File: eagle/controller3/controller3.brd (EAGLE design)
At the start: 68.6 x 63.5 mm, 55 parts, among them J4 USB-MICROB, Q3 MOSFET-NCHANNELFQP30N06L

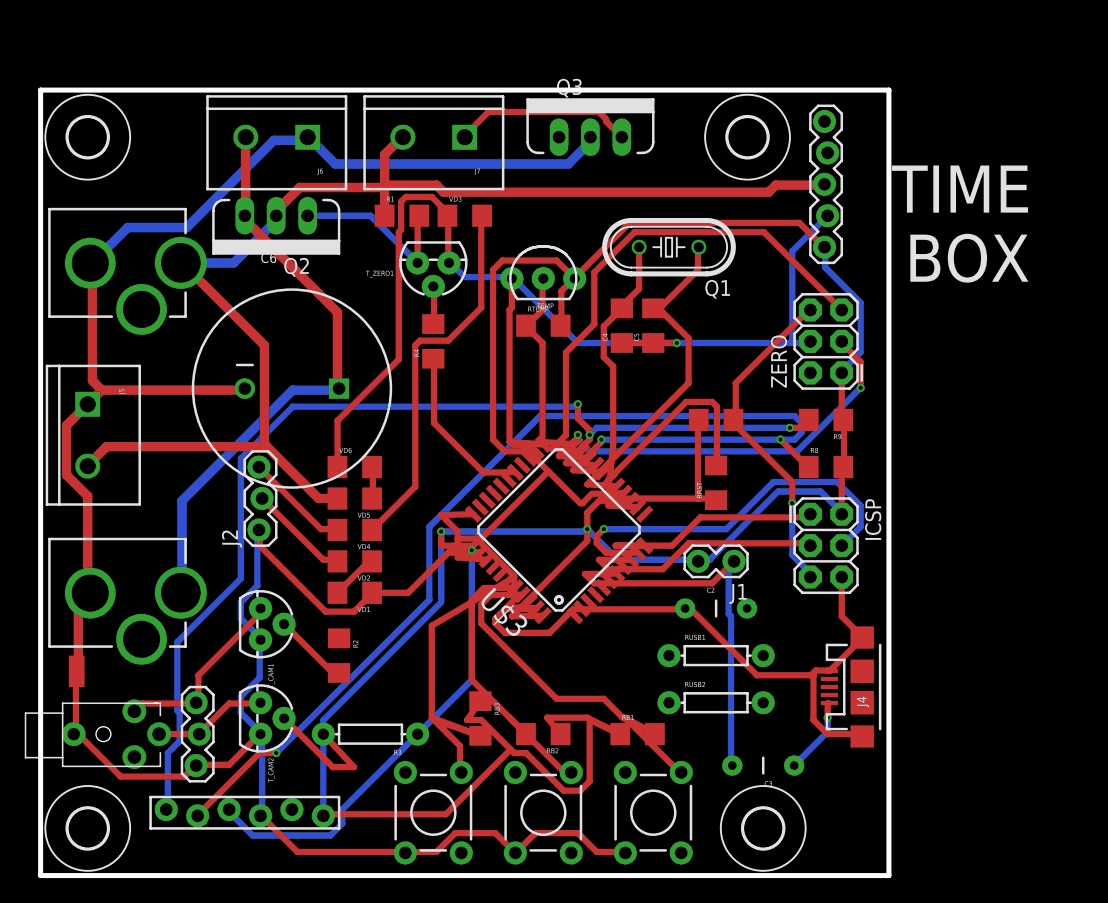
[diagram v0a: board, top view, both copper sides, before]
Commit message: bulk commit (eagle files, old changes)
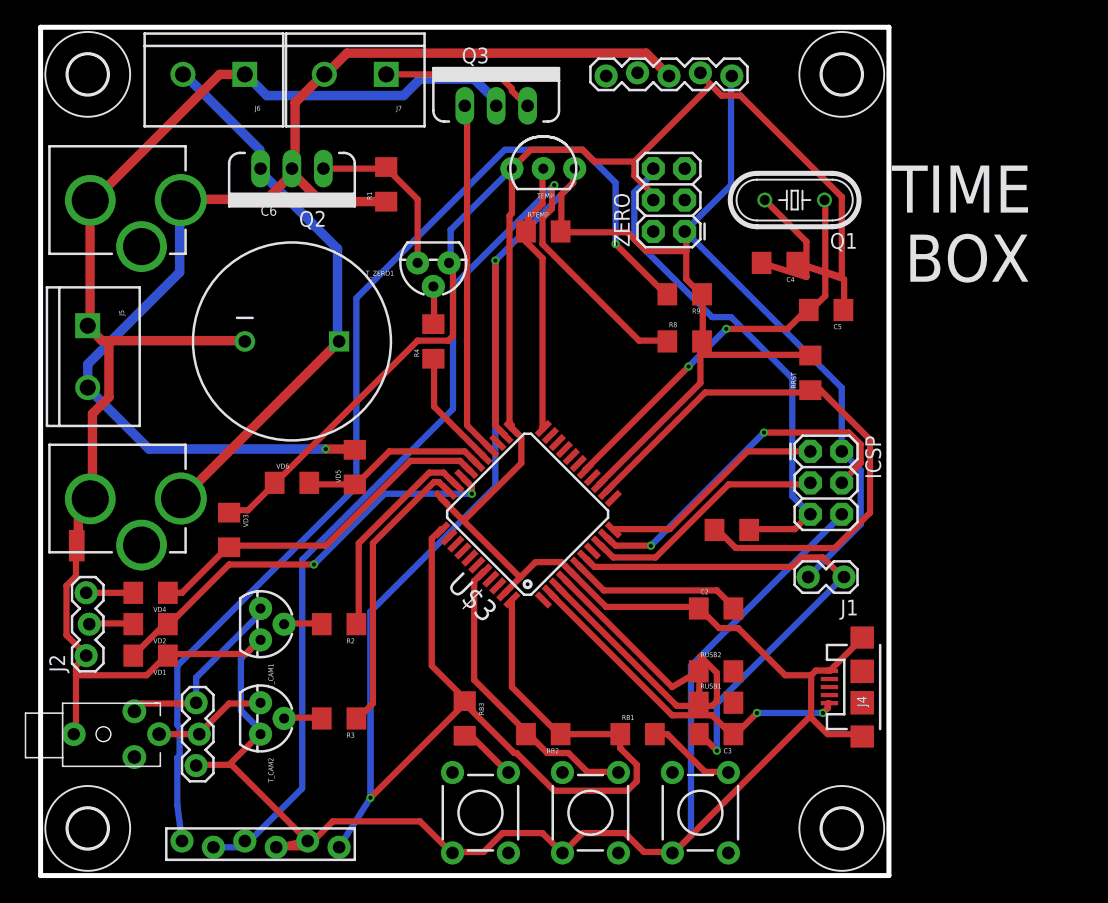
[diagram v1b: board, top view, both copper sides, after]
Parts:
- C2: device SparkFun-Capacitors:CAP-PTH-5MM -> SparkFun-Capacitors:1206
- C3: device SparkFun-Passives:CAP-PTH-5MM -> SparkFun-Passives:1206
- R3, RUSB1, RUSB2: device SparkFun-Passives:AXIAL-0.3 -> SparkFun-Passives:1206
- moved VD3 31.7 mm to (15.2, 27.9), turned to 270 degrees
- moved J2 17.3 mm to (3.81, 17.8)
- moved VD1 17.3 mm to (8.89, 17.8)
- moved VD2 17.3 mm to (8.89, 20.3)
- moved VD4 17.3 mm to (8.89, 22.9)
- moved ZERO 17.1 mm to (52.1, 52.1)
- moved CONV_X_VCC 15.9 mm to (55.9, 64.8), turned to 180 degrees
- moved R9 15.3 mm to (52.1, 47.0)
- moved R8 15.3 mm to (52.1, 43.2)
- moved C5 14.0 mm to (63.5, 45.7), turned to 180 degrees
- moved C4 13.7 mm to (59.7, 49.5), turned to 180 degrees
- moved RRST 11.7 mm to (62.2, 40.6)
- moved Q1 10.9 mm to (61.0, 54.6)
- moved SH 10.2 mm to (2.92, 26.7)
- moved H3 9.16 mm to (64.8, 64.8)
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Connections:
- removed net N$14: J4.D+, RUSB1.P$2
- removed net N$15: J4.D-, RUSB2.P$2
- removed net N$22: C3.1, J4.VBUS
- new net N$12: J4.D-, RUSB1.2
- new net N$13: J4.D+, RUSB2.2
- new net N$6: C3.1, J4.VBUS, U$3.2
- net CAM2: now also R3.1; no longer R3.P$1
- net N$19: now also R3.2; no longer R3.P$2
- net N$4: now also RUSB1.1; no longer RUSB1.P$1
- net N$5: now also RUSB2.1; no longer RUSB2.P$1
- net VCC: no longer U$3.2
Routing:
- net TX: track 42.1 -> 0.00 mm
- net DISP_RST: track 40.7 -> 0.00 mm, vias 1 -> 0
- net RX: track 34.9 -> 0.00 mm, vias 2 -> 0
- net CELL2: track 3.96 -> 34.4 mm, vias 0 -> 2
- net GND: track 294.9 -> 324.0 mm, vias 1 -> 0
- net N$1: track 17.7 -> 46.8 mm
- net EXT_EN: track 0.00 -> 28.7 mm
- net N$6: track 0.00 -> 28.6 mm, vias 0 -> 2
- net N$4: track 0.00 -> 25.0 mm
- net BTN1: track 31.8 -> 7.21 mm
- net CAM2: track 0.00 -> 23.3 mm
- net BTN3: track 27.9 -> 4.79 mm
- net CAM1: track 0.00 -> 17.3 mm
- net N$5: track 0.00 -> 14.8 mm
- net N$20: track 0.00 -> 14.1 mm
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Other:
- board size 68.6 x 63.5 mm -> 68.6 x 68.6 mm
